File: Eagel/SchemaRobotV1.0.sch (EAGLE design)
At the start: 22 parts, among them J1 Connector US1, J2 Connector US 2, J3 Connector US 2, J4 Connector H-Brug, J5 Connector IR voeding, J6 Connector IR signalen, J7 Connector batterij 12v, J8 Connector LCD

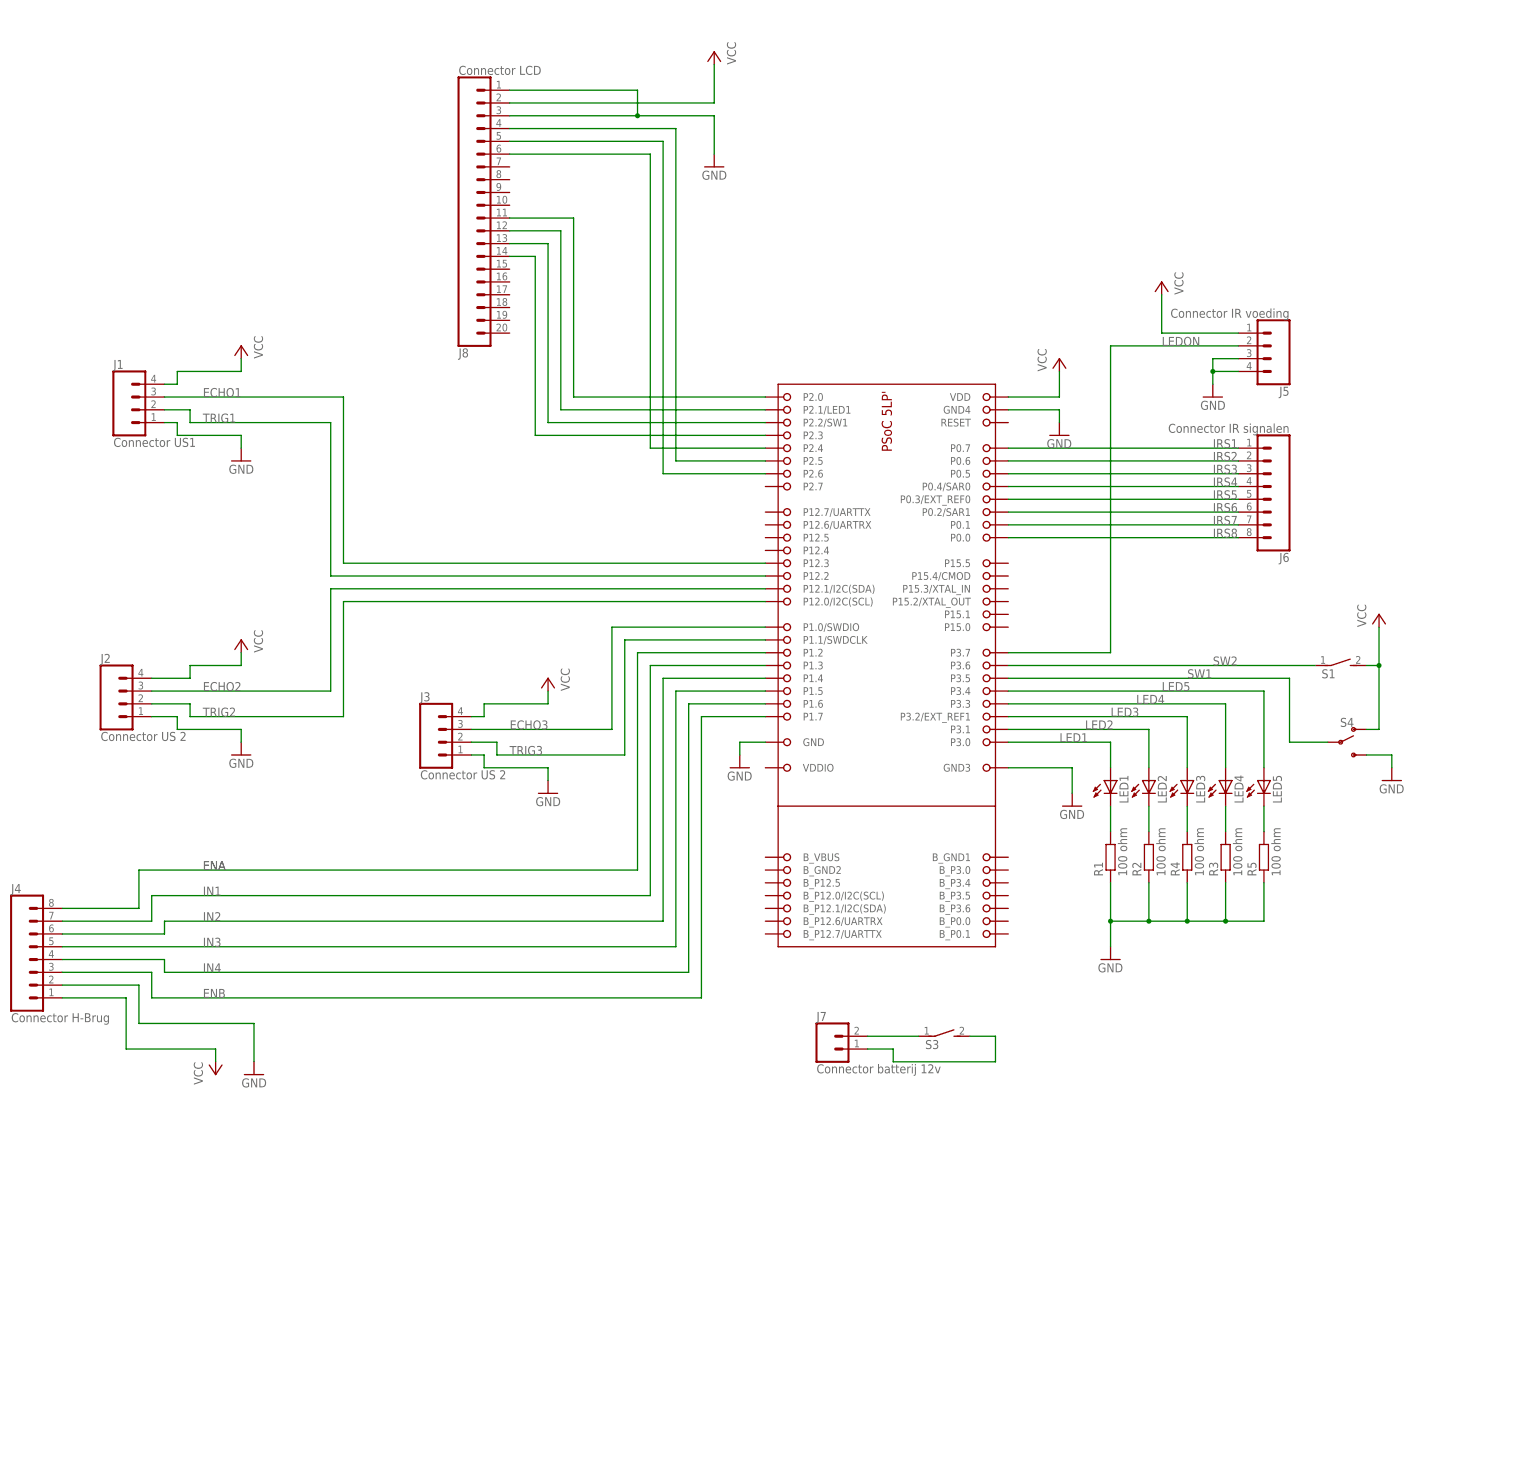
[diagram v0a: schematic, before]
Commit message: eagle
schema klaar, nu pcb nog
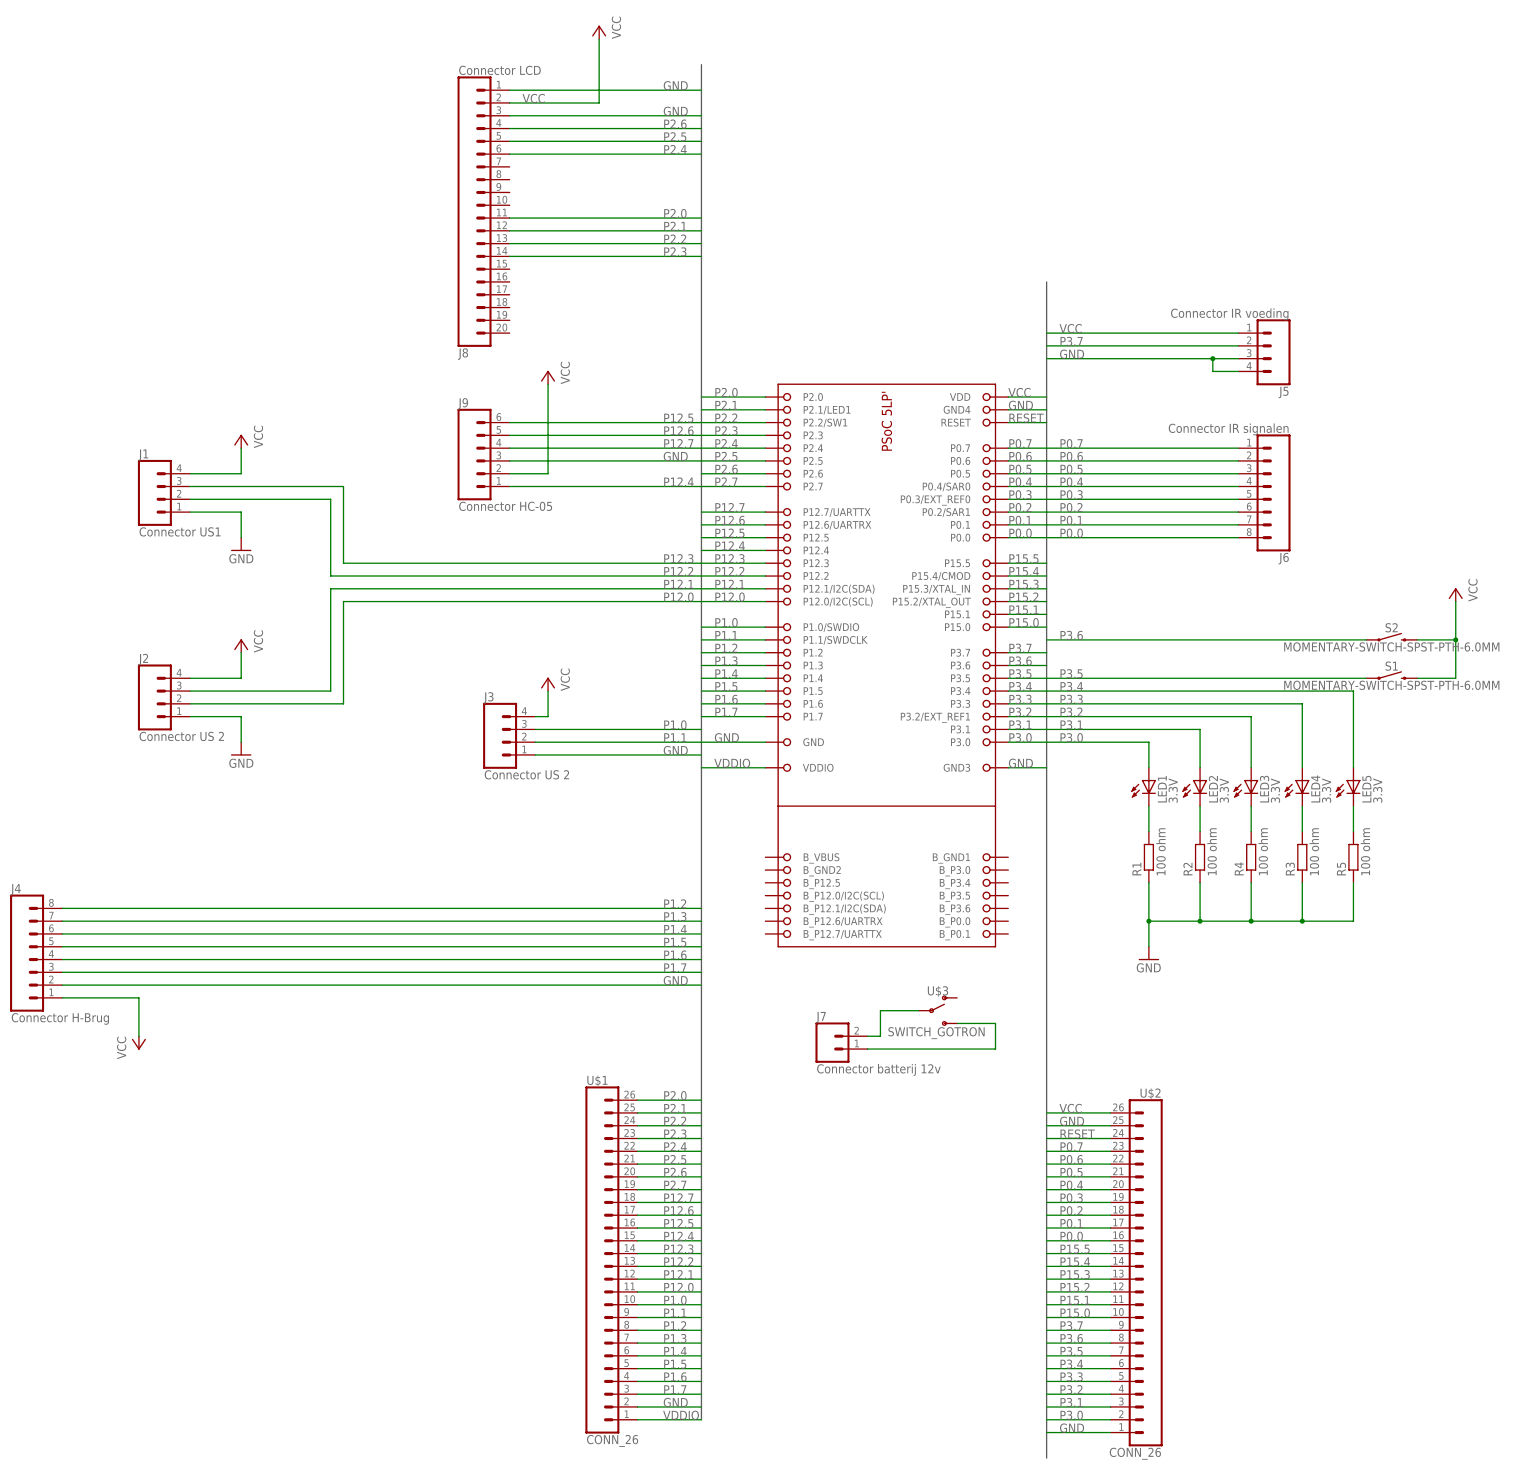
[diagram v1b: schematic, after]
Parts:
- removed S3: (no value), switch-dil:DS01E
- removed S4: (no value), SparkFun-Switches:SWITCH-SPDT-PTH-11.6X4.0MM
- added J9: Connector HC-05, SparkFun-Connectors:CONN_06LOCK
- added S2: MOMENTARY-SWITCH-SPST-PTH-6.0MM, SparkFun-Switches:MOMENTARY-SWITCH-SPST-PTH-6.0MM
- added U$1, U$2: CONN_26, SparkFun-Connectors:CONN_26
- added U$3: SWITCH_GOTRON, SparkFun-Switches:SWITCH_GOTRON
- LED1, LED2, LED3, LED4, LED5: value (none) -> 3.3V
- S1: value (none) -> MOMENTARY-SWITCH-SPST-PTH-6.0MM; device switch-dil:DS01E -> SparkFun-Switches:MOMENTARY-SWITCH-SPST-PTH-6.0MM
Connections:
- removed net ECHO1: DEVICE1.P12.3, J1.3
- removed net ECHO2: DEVICE1.P12.1/I2C(SDA), J2.3
- removed net ECHO3: DEVICE1.P1.0/SWDIO, J3.3
- removed net ENA: DEVICE1.P1.2, J4.8
- removed net ENB: DEVICE1.P1.7, J4.3
- removed net IN1: DEVICE1.P1.3, J4.7
- removed net IN2: DEVICE1.P1.4, J4.6
- removed net IN3: DEVICE1.P1.5, J4.5
- removed net IN4: DEVICE1.P1.6, J4.4
- removed net IRS1: DEVICE1.P0.7, J6.1
- removed net IRS2: DEVICE1.P0.6, J6.2
- removed net IRS3: DEVICE1.P0.5, J6.3
- removed net IRS4: DEVICE1.P0.4/SAR0, J6.4
- removed net IRS5: DEVICE1.P0.3/EXT_REF0, J6.5
- removed net IRS6: DEVICE1.P0.2/SAR1, J6.6
- removed net IRS7: DEVICE1.P0.1, J6.7
- removed net IRS8: DEVICE1.P0.0, J6.8
- removed net LED1: DEVICE1.P3.0, LED1.A
- removed net LED2: DEVICE1.P3.1, LED2.A
- removed net LED3: DEVICE1.P3.2/EXT_REF1, LED3.A
- removed net LED4: DEVICE1.P3.3, LED4.A
- removed net LED5: DEVICE1.P3.4, LED5.A
- removed net LEDON: DEVICE1.P3.7, J5.2
- removed net N$10: DEVICE1.P2.4, J8.6
- removed net N$11: DEVICE1.P2.6, J8.5
- removed net N$12: DEVICE1.P2.5, J8.4
- removed net N$13: J7.2, S3.1
- removed net N$14: J7.1, S3.2
- removed net N$8: DEVICE1.P2.1/LED1, J8.12
- removed net N$9: DEVICE1.P2.0, J8.11
- removed net SW1: DEVICE1.P3.5, S4.P
- removed net SW2: DEVICE1.P3.6, S1.1
- removed net TRIG1: DEVICE1.P12.2, J1.2
- removed net TRIG2: DEVICE1.P12.0/I2C(SCL), J2.2
- removed net TRIG3: DEVICE1.P1.1/SWDCLK, J3.2
- new net P0.0: DEVICE1.P0.0, J6.8, U$2.16
- new net P0.1: DEVICE1.P0.1, J6.7, U$2.17
- new net P0.2: DEVICE1.P0.2/SAR1, J6.6, U$2.18
- new net P0.3: DEVICE1.P0.3/EXT_REF0, J6.5, U$2.19
- new net P0.4: DEVICE1.P0.4/SAR0, J6.4, U$2.20
- new net P0.5: DEVICE1.P0.5, J6.3, U$2.21
- new net P0.6: DEVICE1.P0.6, J6.2, U$2.22
- new net P0.7: DEVICE1.P0.7, J6.1, U$2.23
- new net P1.0: DEVICE1.P1.0/SWDIO, J3.3, U$1.10
- new net P1.1: DEVICE1.P1.1/SWDCLK, J3.2, U$1.9
- new net P1.2: DEVICE1.P1.2, J4.8, U$1.8
- new net P1.3: DEVICE1.P1.3, J4.7, U$1.7
- new net P1.4: DEVICE1.P1.4, J4.6, U$1.6
- new net P1.5: DEVICE1.P1.5, J4.5, U$1.5
- new net P1.6: DEVICE1.P1.6, J4.4, U$1.4
- new net P1.7: DEVICE1.P1.7, J4.3, U$1.3
- new net P12.0: DEVICE1.P12.0/I2C(SCL), J2.2, U$1.11
- new net P12.1: DEVICE1.P12.1/I2C(SDA), J2.3, U$1.12
- new net P12.2: DEVICE1.P12.2, J1.2, U$1.13
- new net P12.3: DEVICE1.P12.3, J1.3, U$1.14
- new net P12.4: DEVICE1.P12.4, J9.1, U$1.15
- new net P12.5: DEVICE1.P12.5, J9.6, U$1.16
- new net P12.6: DEVICE1.P12.6/UARTRX, J9.5, U$1.17
- new net P12.7: DEVICE1.P12.7/UARTTX, J9.4, U$1.18
- new net P15.0: DEVICE1.P15.0, U$2.10
- new net P15.1: DEVICE1.P15.1, U$2.11
- new net P15.2: DEVICE1.P15.2/XTAL_OUT, U$2.12
- new net P15.3: DEVICE1.P15.3/XTAL_IN, U$2.13
- new net P15.4: DEVICE1.P15.4/CMOD, U$2.14
- new net P15.5: DEVICE1.P15.5, U$2.15
- new net P2.0: DEVICE1.P2.0, J8.11, U$1.26
- new net P2.1: DEVICE1.P2.1/LED1, J8.12, U$1.25
- new net P2.2: DEVICE1.P2.2/SW1, J8.13, U$1.24
- new net P2.3: DEVICE1.P2.3, J8.14, U$1.23
- new net P2.4: DEVICE1.P2.4, J8.6, U$1.22
- new net P2.5: DEVICE1.P2.5, J8.4, U$1.21
- new net P2.6: DEVICE1.P2.6, J8.5, U$1.20
- new net P2.7: DEVICE1.P2.7, U$1.19
- new net P3.0: DEVICE1.P3.0, LED1.A, U$2.2
- new net P3.1: DEVICE1.P3.1, LED2.A, U$2.3
- new net P3.2: DEVICE1.P3.2/EXT_REF1, LED3.A, U$2.4
- new net P3.3: DEVICE1.P3.3, LED4.A, U$2.5
- new net P3.4: DEVICE1.P3.4, LED5.A, U$2.6
- new net P3.5: DEVICE1.P3.5, S1.1, U$2.7
- new net P3.6: DEVICE1.P3.6, S2.1, U$2.8
- new net P3.7: DEVICE1.P3.7, J5.2, U$2.9
- new net RESET: DEVICE1.RESET, U$2.24
- new net VDDIO: DEVICE1.VDDIO, U$1.1
- net GND: now also J9.3, U$1.2, U$2.1, U$2.25; no longer S4.S
- net N$1: now also J7.2, U$3.P; no longer DEVICE1.P2.3, J8.14
- net N$7: now also J7.1, U$3.S; no longer DEVICE1.P2.2/SW1, J8.13
- net VCC: now also J9.2, S2.2, U$2.26; no longer S4.O
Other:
- moved on the sheet: J1, J2, J3, LED1, LED2, LED3, LED4, LED5, R1, R2, R3, R4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

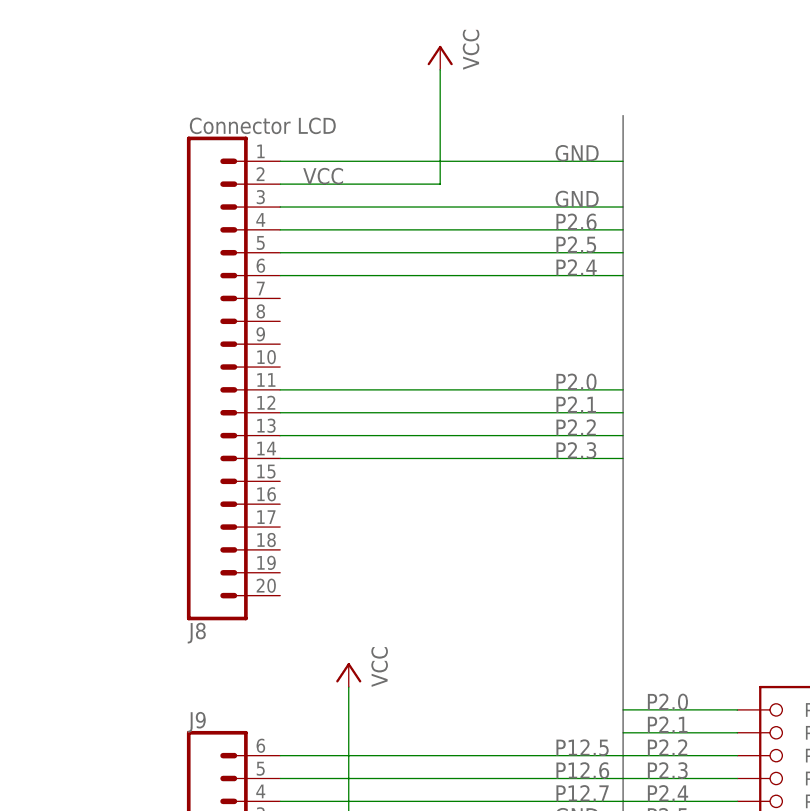
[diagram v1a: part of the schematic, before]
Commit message: eagle
pcb bijna af
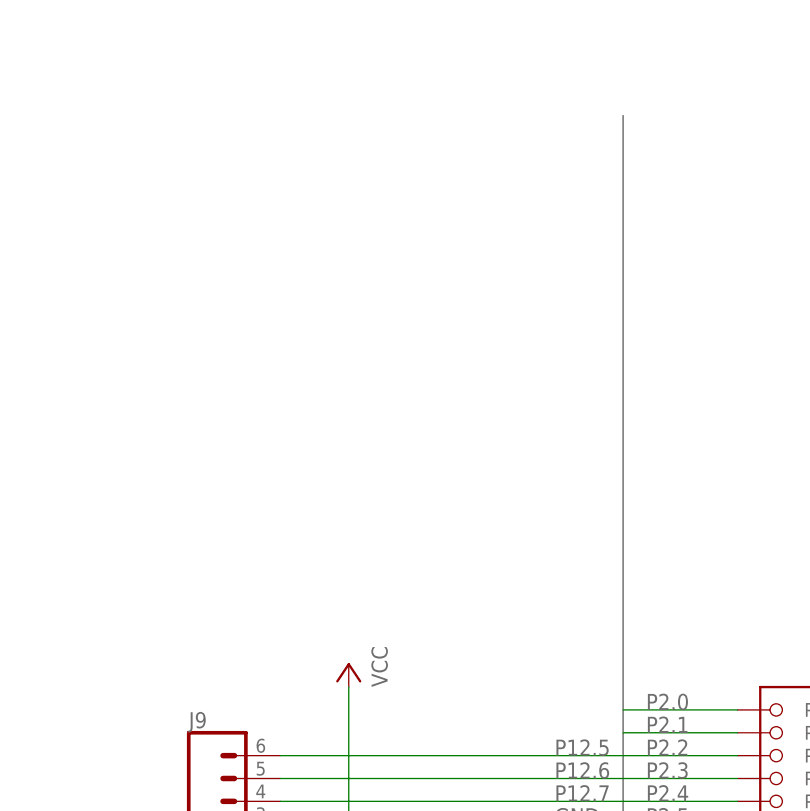
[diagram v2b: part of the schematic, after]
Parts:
- removed J8: Connector LCD, SparkFun-Connectors:CONN_20
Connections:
- net GND: no longer J8.1, J8.3
- net P2.0: no longer J8.11
- net P2.1: no longer J8.12
- net P2.2: no longer J8.13
- net P2.3: no longer J8.14
- net P2.4: no longer J8.6
- net P2.5: no longer J8.4
- net P2.6: no longer J8.5
- net VCC: no longer J8.2
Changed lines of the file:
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@@
 <part name="J6" library="SparkFun-Connectors" library_urn="urn:adsk.eagle:library:513" deviceset="CONN_08" device="3.5MM-8" package3d_urn="urn:adsk.eagle:package:38143/1" value="Connector IR signalen"/>
 <part name="J7" library="SparkFun-Connectors" library_urn="urn:adsk.eagle:library:513" deviceset="CONN_02" device="3.5MM" package3d_urn="urn:adsk.eagle:package:38050/1" value="Connector batterij 12v"/>
-<part name="J8" library="SparkFun-Connectors" library_urn="urn:adsk.eagle:library:513" deviceset="CONN_20" device="" package3d_urn="urn:adsk.eagle:package:38196/1" value="Connector LCD"/>
 <part name="U$1" library="SparkFun-Connectors" deviceset="CONN_26" device=""/>
 <part name="U$2" library="SparkFun-Connectors" deviceset="CONN_26" device=""/>
-<part name="P+6" library="supply1" library_urn="urn:adsk.eagle:library:371" deviceset="VCC" device=""/>
 <part name="J9" library="SparkFun-Connectors" deviceset="CONN_06" device="LOCK" value="Connector HC-05"/>
 <part name="P+4" library="supply1" library_urn="urn:adsk.eagle:library:371" deviceset="VCC" device=""/>
@@
 <instance part="J6" gate="G$1" x="132.08" y="119.38" rot="R180"/>
 <instance part="J7" gate="G$1" x="45.72" y="7.62"/>
-<instance part="J8" gate="G$1" x="-27.94" y="203.2" rot="MR180"/>
 <instance part="U$1" gate="G$1" x="-2.54" y="-33.02"/>
 <instance part="U$2" gate="G$1" x="111.76" y="-35.56" rot="MR0"/>
-<instance part="P+6" gate="VCC" x="0" y="210.82" rot="MR0"/>
 <instance part="J9" gate="G$1" x="-22.86" y="124.46"/>
 <instance part="P+4" gate="VCC" x="-10.16" y="142.24" rot="MR0"/>
@@
 </segment>
 <segment>
-<pinref part="J8" gate="G$1" pin="1"/>
-<wire x1="-17.78" y1="198.12" x2="20.32" y2="198.12" width="0.1524" layer="91"/>
-<label x="12.7" y="198.12" size="1.778" layer="95"/>
-</segment>
-<segment>
-<pinref part="J8" gate="G$1" pin="3"/>
-<wire x1="20.32" y1="193.04" x2="-17.78" y2="193.04" width="0.1524" layer="91"/>
-<label x="12.7" y="193.04" size="1.778" layer="95"/>
-</segment>
-<segment>
 <pinref part="J3" gate="G$1" pin="1"/>
 <wire x1="20.32" y1="66.04" x2="-12.7" y2="66.04" width="0.1524" layer="91"/>
@@
 </segment>
 <segment>
-<pinref part="J8" gate="G$1" pin="2"/>
-<wire x1="-17.78" y1="195.58" x2="0" y2="195.58" width="0.1524" layer="91"/>
-<wire x1="0" y1="195.58" x2="0" y2="208.28" width="0.1524" layer="91"/>
-<pinref part="P+6" gate="VCC" pin="VCC"/>
-<label x="-15.24" y="195.58" size="1.778" layer="95"/>
-</segment>
-<segment>
 <pinref part="DEVICE1" gate="G$1" pin="VDD"/>
 <wire x1="88.9" y1="137.16" x2="81.28" y2="137.16" width="0.1524" layer="91"/>
@@
 <net name="P2.3" class="0">
 <segment>
-<pinref part="J8" gate="G$1" pin="14"/>
-<label x="12.7" y="165.1" size="1.778" layer="95"/>
-<wire x1="-17.78" y1="165.1" x2="20.32" y2="165.1" width="0.1524" layer="91"/>
-</segment>
-<segment>
 <pinref part="DEVICE1" gate="G$1" pin="P2.3"/>
 <wire x1="33.02" y1="129.54" x2="20.32" y2="129.54" width="0.1524" layer="91"/>
@@
 <net name="P2.2" class="0">
 <segment>
-<pinref part="J8" gate="G$1" pin="13"/>
-<label x="12.7" y="167.64" size="1.778" layer="95"/>
-<wire x1="-17.78" y1="167.64" x2="20.32" y2="167.64" width="0.1524" layer="91"/>
-</segment>
-<segment>
 <pinref part="DEVICE1" gate="G$1" pin="P2.2/SW1"/>
 <wire x1="33.02" y1="132.08" x2="20.32" y2="132.08" width="0.1524" layer="91"/>
@@
 <net name="P2.1" class="0">
 <segment>
-<pinref part="J8" gate="G$1" pin="12"/>
-<label x="12.7" y="170.18" size="1.778" layer="95"/>
-<wire x1="-17.78" y1="170.18" x2="20.32" y2="170.18" width="0.1524" layer="91"/>
-</segment>
-<segment>
 <pinref part="DEVICE1" gate="G$1" pin="P2.1/LED1"/>
 <wire x1="33.02" y1="134.62" x2="20.32" y2="134.62" width="0.1524" layer="91"/>
@@
 <net name="P2.0" class="0">
 <segment>
-<pinref part="J8" gate="G$1" pin="11"/>
-<label x="12.7" y="172.72" size="1.778" layer="95"/>
-<wire x1="-17.78" y1="172.72" x2="20.32" y2="172.72" width="0.1524" layer="91"/>
-</segment>
-<segment>
 <pinref part="DEVICE1" gate="G$1" pin="P2.0"/>
 <wire x1="33.02" y1="137.16" x2="20.32" y2="137.16" width="0.1524" layer="91"/>
@@
 <net name="P2.4" class="0">
 <segment>
-<pinref part="J8" gate="G$1" pin="6"/>
-<wire x1="-17.78" y1="185.42" x2="20.32" y2="185.42" width="0.1524" layer="91"/>
-<label x="12.7" y="185.42" size="1.778" layer="95"/>
-</segment>
-<segment>
 <pinref part="DEVICE1" gate="G$1" pin="P2.4"/>
 <wire x1="33.02" y1="127" x2="20.32" y2="127" width="0.1524" layer="91"/>
@@
 <net name="P2.6" class="0">
 <segment>
-<pinref part="J8" gate="G$1" pin="5"/>
-<wire x1="-17.78" y1="187.96" x2="20.32" y2="187.96" width="0.1524" layer="91"/>
-<label x="12.7" y="190.5" size="1.778" layer="95"/>
-</segment>
-<segment>
 <pinref part="DEVICE1" gate="G$1" pin="P2.6"/>
 <wire x1="33.02" y1="121.92" x2="20.32" y2="121.92" width="0.1524" layer="91"/>
@@
 </net>
 <net name="P2.5" class="0">
-<segment>
-<pinref part="J8" gate="G$1" pin="4"/>
-<wire x1="-17.78" y1="190.5" x2="20.32" y2="190.5" width="0.1524" layer="91"/>
-<label x="12.7" y="187.96" size="1.778" layer="95"/>
-</segment>
 <segment>
 <pinref part="DEVICE1" gate="G$1" pin="P2.5"/>
@@
 </sheet>
 </sheets>
-<errors>
-</errors>
 </schematic>
 </drawing>
